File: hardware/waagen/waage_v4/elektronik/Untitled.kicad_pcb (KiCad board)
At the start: 2 copper layers, 103.2 x 17.8 mm, 9 parts, among them J1 USB_A, J2 Conn_01x03, J3 USB_A, SW1 SW_Push, U1 ATtiny414-SS

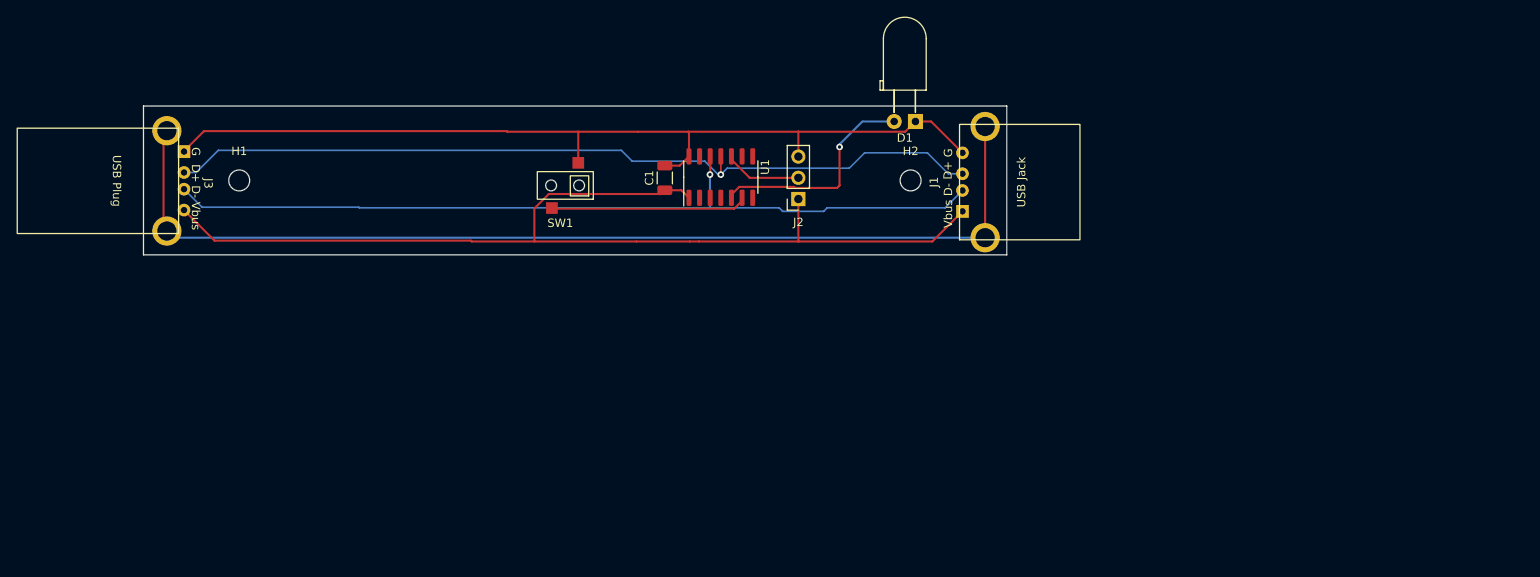
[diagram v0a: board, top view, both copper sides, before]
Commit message: intermediate step
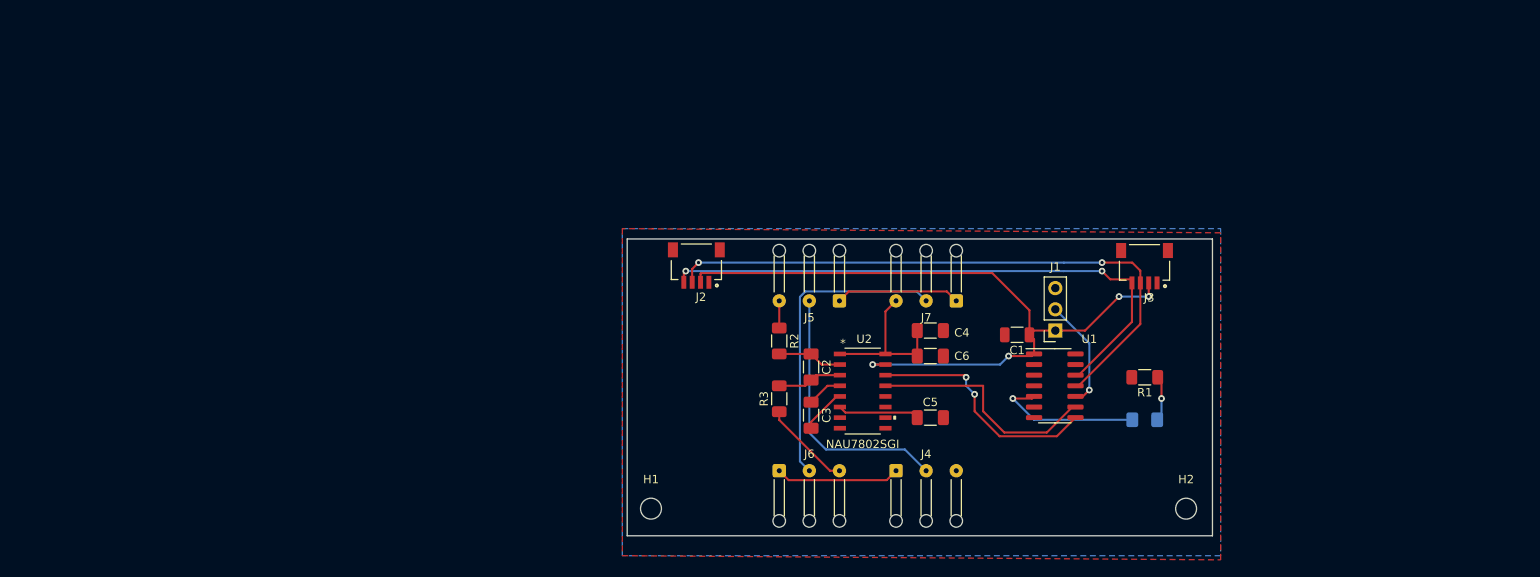
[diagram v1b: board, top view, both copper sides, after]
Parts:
- removed SW1: SW_Push, Library_USB_A:Button_Switch_ESE-11MV1T
- added C2: 100n, Capacitor_SMD:C_1206_3216Metric_Pad1.33x1.80mm_HandSolder, F.Cu at (142.0, 96.8)
- added C3: 330p, Capacitor_SMD:C_1206_3216Metric_Pad1.33x1.80mm_HandSolder, F.Cu at (142.0, 102.6)
- added C4: 1µ, Capacitor_SMD:C_1206_3216Metric_Pad1.33x1.80mm_HandSolder, F.Cu at (156.3, 92.5)
- added C5: 100n, Capacitor_SMD:C_1206_3216Metric_Pad1.33x1.80mm_HandSolder, F.Cu at (156.3, 102.9)
- added C6: 100n, Capacitor_SMD:C_1206_3216Metric_Pad1.33x1.80mm_HandSolder, F.Cu at (156.3, 95.5)
- added J4: Conn_01x03_Male, Connector_Wire:SolderWire-0.1sqmm_1x03_P3.6mm_D0.4mm_OD1mm_Relief, F.Cu at (152.2, 109.2)
- added J5: Conn_01x03_Male, Connector_Wire:SolderWire-0.1sqmm_1x03_P3.6mm_D0.4mm_OD1mm_Relief, F.Cu at (145.4, 88.9)
- added J6: Conn_01x03_Male, Connector_Wire:SolderWire-0.1sqmm_1x03_P3.6mm_D0.4mm_OD1mm_Relief, F.Cu at (138.2, 109.2)
- added J7: Conn_01x03_Male, Connector_Wire:SolderWire-0.1sqmm_1x03_P3.6mm_D0.4mm_OD1mm_Relief, F.Cu at (159.4, 88.9)
- added R1: 180, Resistor_SMD:R_1206_3216Metric_Pad1.30x1.75mm_HandSolder, F.Cu at (181.9, 98.0)
- added R2: 47, Resistor_SMD:R_1206_3216Metric_Pad1.30x1.75mm_HandSolder, F.Cu at (138.2, 93.7)
- added R3: 47, Resistor_SMD:R_1206_3216Metric_Pad1.30x1.75mm_HandSolder, F.Cu at (138.2, 100.6)
- added U2: NAU7802SGI, NAU:NAU7802SGI, F.Cu at (148.2, 99.7)
- D1: footprint LED_THT:LED_D5.0mm_Horizontal_O3.81mm_Z9.0mm -> LED_SMD:LED_1206_3216Metric_Pad1.42x1.75mm_HandSolder; moved to B.Cu
- J1: value USB_A -> Conn_01x03; footprint Library_USB_A:Conn_USB_A_Jack -> Connector_PinSocket_2.54mm:PinSocket_1x03_P2.54mm_Vertical
- J2: value Conn_01x03 -> SM04B-SRSS-TB(LF)(SN); footprint Connector_PinSocket_2.54mm:PinSocket_1x03_P2.54mm_Vertical -> Quiicconnector:JST_SM04B-SRSS-TB(LF)(SN)
- J3: value USB_A -> SM04B-SRSS-TB(LF)(SN); footprint Library_USB_A:Conn_USB_A_Plug -> Quiicconnector:JST_SM04B-SRSS-TB(LF)(SN)
- U1: value ATtiny414-SS -> ATtiny1614-SS
- moved J3 115.5 mm to (181.9, 86.8), turned to 180 degrees
- moved H1 63.0 mm to (122.8, 113.8)
- moved H2 51.3 mm to (186.8, 113.8)
- moved U1 47.1 mm to (171.1, 99.1), turned to 0 degrees
- moved C1 46.1 mm to (166.6, 93.0), turned to 180 degrees
- moved D1 45.0 mm to (181.9, 103.1)
- moved J1 20.9 mm to (171.2, 92.5), turned to 180 degrees
- moved J2 15.7 mm to (128.3, 86.7)
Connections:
- D1 pad 1: GND -> Net-(D1-K)
- J1 pad 2: Data- -> Net-(J1-Pin_2)
- J1 pad 3: Data+ -> GND
- J2 pad 1: VCC -> GND
- J2 pad 2: Net-(J2-Pad2) -> VCC
- J2 pad 3: GND -> SDA_1
- J3 pad 1: VCC -> GND
- J3 pad 2: Data- -> VCC
- J3 pad 3: Data+ -> SDA_1
- J3 pad 4: GND -> SCL_1
- U1 pad 10: Net-(J2-Pad2) -> Net-(J1-Pin_2)
- U1 pad 11: Data+ -> SDA_1
- U1 pad 12: Data- -> SCL_1
- U1 pad 6: Net-(SW1-Pad2) -> unconnected-(U1-PB3-Pad6)
- U1 pad 8: unconnected-(U1-Pad8) -> /SDA_0
- U1 pad 9: unconnected-(U1-Pad9) -> /SCL_0
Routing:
- net Net-(J1-Pad5): track 123.5 -> 0.00 mm
- net GND: track 109.3 -> 0.00 mm
- net Data-: track 101.3 -> 0.00 mm, vias 1 -> 0
- net Data+: track 99.7 -> 0.00 mm, vias 1 -> 0
- net SDA_1: track 0.00 -> 73.1 mm, vias 0 -> 2
- net SCL_1: track 0.00 -> 69.7 mm, vias 0 -> 2
- net VCC: track 124.9 -> 87.3 mm, vias 0 -> 4
- net Net-(J6-Pin_2): track 0.00 -> 37.1 mm
- net Net-(J4-Pin_2): track 0.00 -> 31.6 mm
- net /SDA_0: track 0.00 -> 28.5 mm, vias 0 -> 2
- net /SCL_0: track 0.00 -> 28.1 mm
- net Net-(SW1-Pad2): track 23.5 -> 0.00 mm
- net /Scale/NAU_VDDA: track 0.00 -> 19.9 mm
- net Net-(J5-Pin_1): track 0.00 -> 14.9 mm
- net Net-(J4-Pin_1): track 0.00 -> 14.9 mm
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- added copper zone on B.Cu, net GND
- added copper zone on F.Cu, net GND
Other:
- board size 103.2 x 17.8 mm -> 70 x 35.5 mm

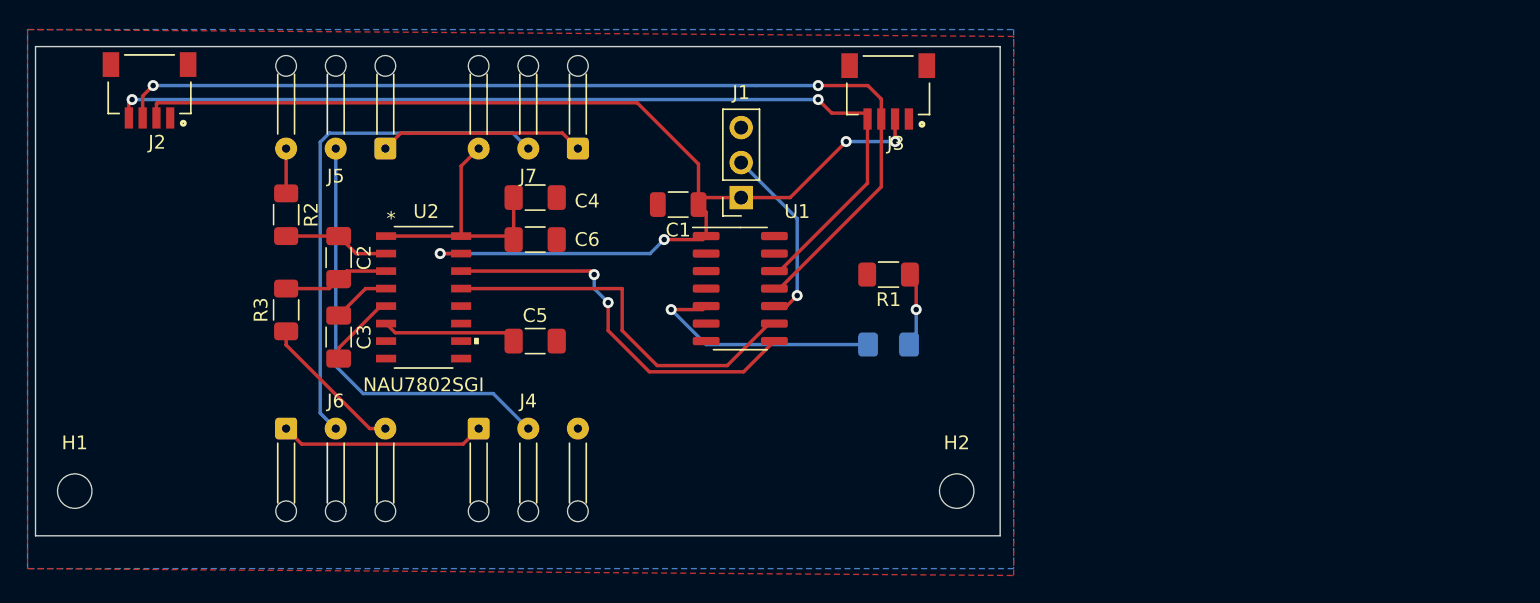
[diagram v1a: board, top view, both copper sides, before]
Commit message: Zwischenstand Elektronik v4
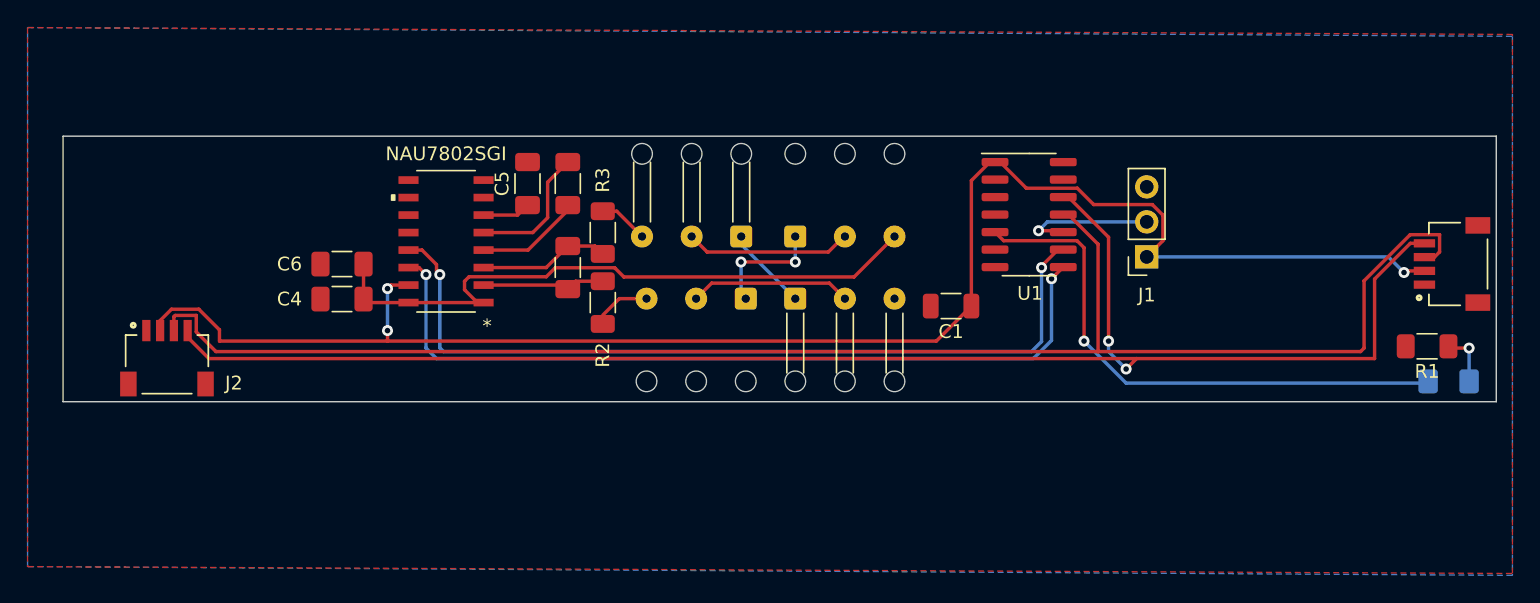
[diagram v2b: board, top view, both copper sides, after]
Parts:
- removed H1, H2: MountingHole, MountingHole:MountingHole_2.5mm
- J5, J7: moved to B.Cu
- moved D1 40.7 mm to (222.5, 105.8)
- moved J3 40.3 mm to (220.8, 97.3), turned to 90 degrees
- moved R1 39.4 mm to (221.0, 103.3)
- moved J6 35.8 mm to (171.2, 95.3), turned to 180 degrees
- moved J1 29.7 mm to (200.6, 96.8)
- moved J5 28.3 mm to (171.5, 99.8)
- moved J4 24.8 mm to (175.1, 99.8)
- moved R2 23.8 mm to (161.2, 100.1), turned to 90 degrees
- moved R3 23.7 mm to (161.2, 95.0), turned to -90 degrees
- moved U1 21.6 mm to (192.1, 93.7)
- moved C1 21.1 mm to (186.4, 100.3)
- moved C3 20.0 mm to (158.6, 91.4), turned to 90 degrees
- moved J7 17.0 mm to (175.1, 95.3), turned to 0 degrees
- moved C2 16.6 mm to (158.6, 97.5), turned to 90 degrees
- moved C4 15.8 mm to (142.2, 99.8), turned to 180 degrees
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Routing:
- net SCL_1: track 69.7 -> 113.4 mm
- net SDA_1: track 73.1 -> 114.8 mm, vias 2 -> 0
- net /SCL_0: track 28.1 -> 60.2 mm, vias 0 -> 2
- net /SDA_0: track 28.5 -> 58.7 mm
- net VCC: track 87.3 -> 117.2 mm, vias 4 -> 3
- net /Scale/NAU_VDDA: track 19.9 -> 46.8 mm
- net Net-(J6-Pin_2): track 37.1 -> 12.2 mm
- net Net-(D1-A): track 18.0 -> 40.0 mm
- net Net-(J4-Pin_2): track 31.6 -> 11.7 mm
- net Net-(J4-Pin_1): track 14.9 -> 6.13 mm
- net Net-(J6-Pin_3): track 10.7 -> 3.61 mm
- net Net-(J5-Pin_1): track 14.9 -> 8.59 mm, vias 0 -> 2
- net Net-(U2-VBG): track 9.78 -> 3.49 mm
- net Net-(U2-VIN2P): track 5.46 -> 9.74 mm
- net Net-(J1-Pin_2): track 13.3 -> 9.95 mm
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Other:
- board size 70 x 35.5 mm -> 104 x 19.3 mm
